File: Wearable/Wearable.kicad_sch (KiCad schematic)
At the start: 6 parts, among them P1 USB_C_Plug, U1 w, U2 MAX30102, U3 MAX30205MTA+, U4 ICM-42605, U5 MAX30003CTI+T

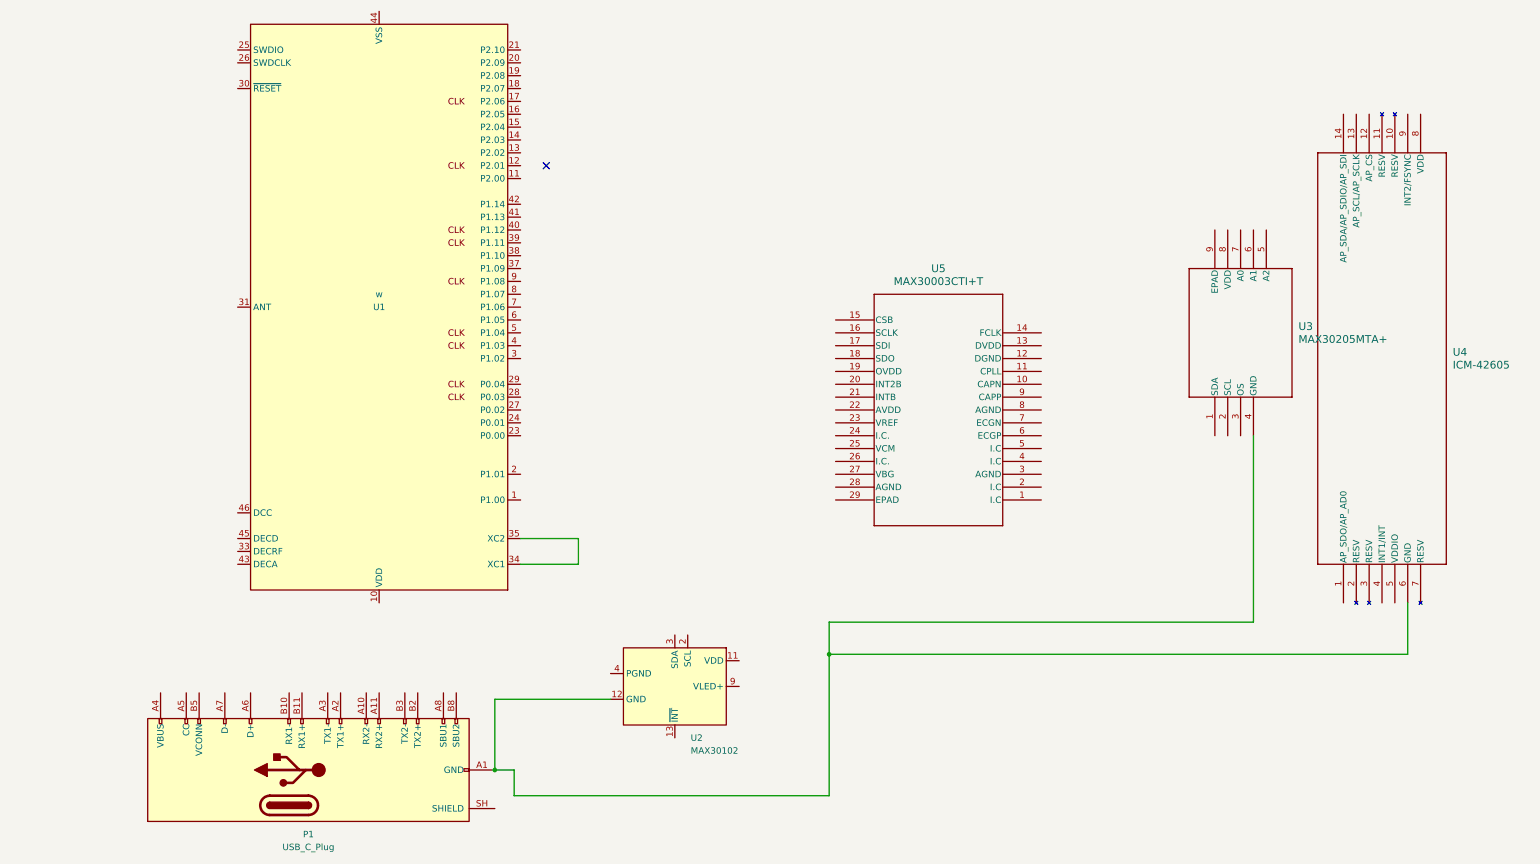
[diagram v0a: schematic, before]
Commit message: Added much more wiring,Good progress
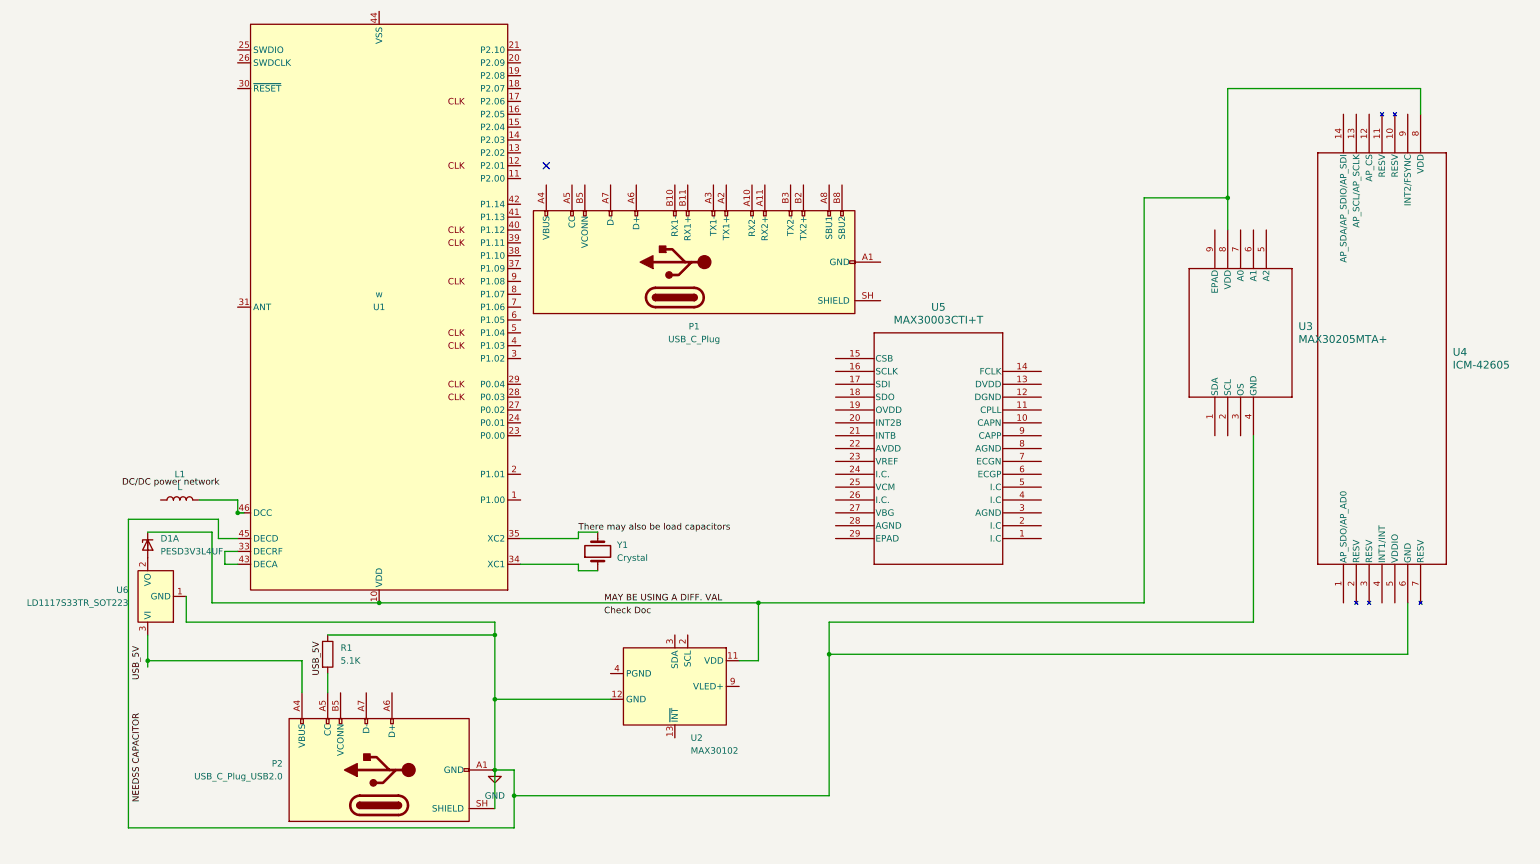
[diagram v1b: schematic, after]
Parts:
- added D1: PESD3V3L4UF, Package_TO_SOT_SMD:SOT-886, symbol Power_Protection:PESD3V3L4UF
- added L1: L, symbol Device:L
- added P2: USB_C_Plug_USB2.0, symbol Connector:USB_C_Plug_USB2.0
- added R1: 5.1K, symbol Device:R
- added U6: LD1117S33TR_SOT223, Package_TO_SOT_SMD:SOT-223-3_TabPin2, symbol Regulator_Linear:LD1117S33TR_SOT223
- added Y1: Crystal, symbol Device:Crystal
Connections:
- net at P1.A1 (GND), P1.A12 (GND), P1.B1 (GND)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: no longer U2.12 (GND), U3.4 (GND), U4.6 (GND)
- net MAY BE USING A DIFF. VAL: now reaches U4.8 (VDD)
- net MAY BE USING A DIFF. VAL: now also U1.10 (VDD), U1.22 (VDD), U1.36 (VDD), U1.47 (VDD), U1.48 (VDD), U2.11 (VDD), U3.8 (VDD), D1.1 (K1)
- net at U1.33 (DECRF): now also U1.43 (DECA)
- net at U1.34 (XC1): now also Y1.1; no longer U1.35 (XC2)
- net GND: now reaches U1.45 (DECD)
- net GND: now also U2.12 (GND), U3.4 (GND), U4.6 (GND), P2.A1 (GND), P2.A12 (GND), P2.B1 (GND), P2.B12 (GND), P2.SH (SHIELD), R1.1, U6.1 (GND)
- net at U1.46 (DCC): now also L1.2
- new net: D1.2 (A), D1.5 (A), U6.2 (VO)
- new net: P2.A4 (VBUS), P2.A9 (VBUS), P2.B4 (VBUS), P2.B9 (VBUS), U6.3 (VI)
- new net: P2.A5 (CC), R1.2
- new net There may also be load capacitors: U1.35 (XC2), Y1.2
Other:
- moved on the sheet: P1, U5
